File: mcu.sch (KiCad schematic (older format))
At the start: 12 parts, among them J501 JTAG, J502 Serial / Bootloader, SW501 EVQQ2, SW502 EVQQ2, U501 STM32F405RGTx, Y501 8MHz

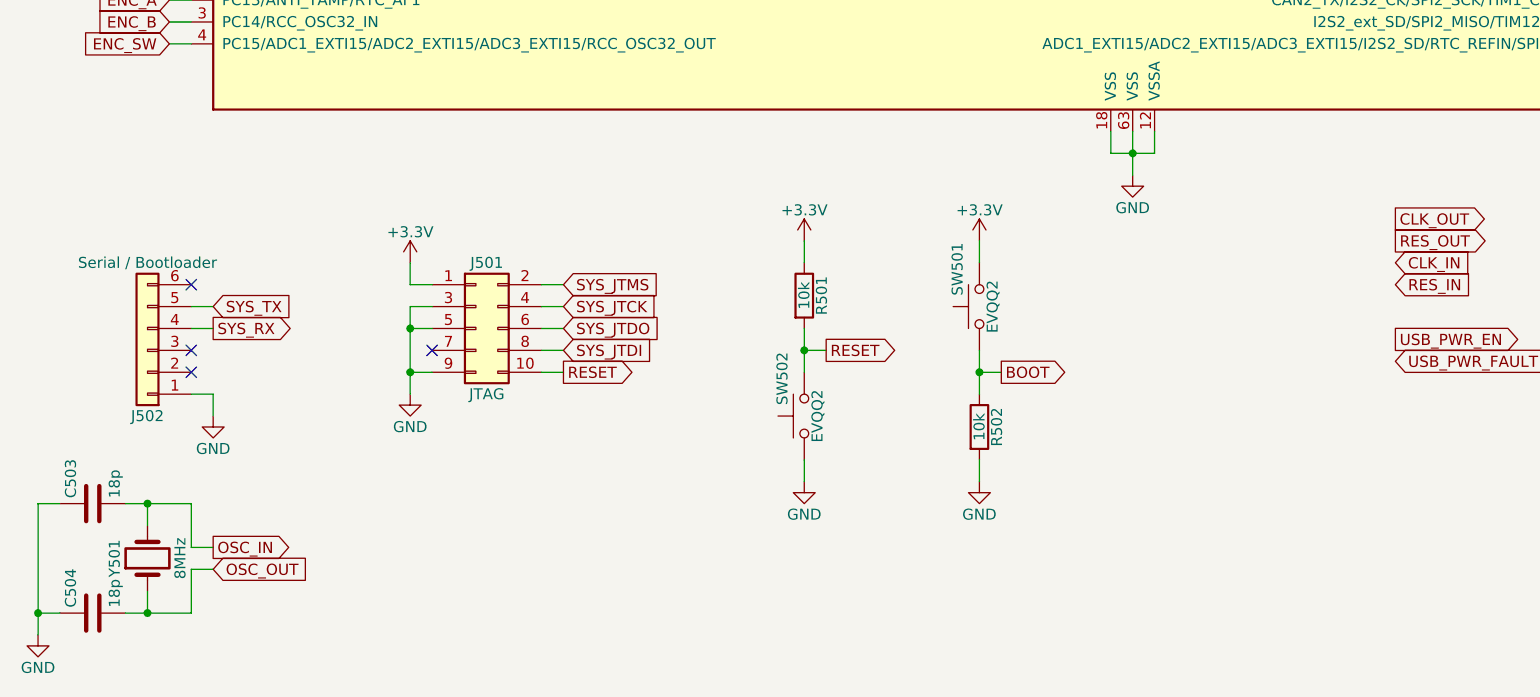
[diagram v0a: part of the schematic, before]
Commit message: work in progress
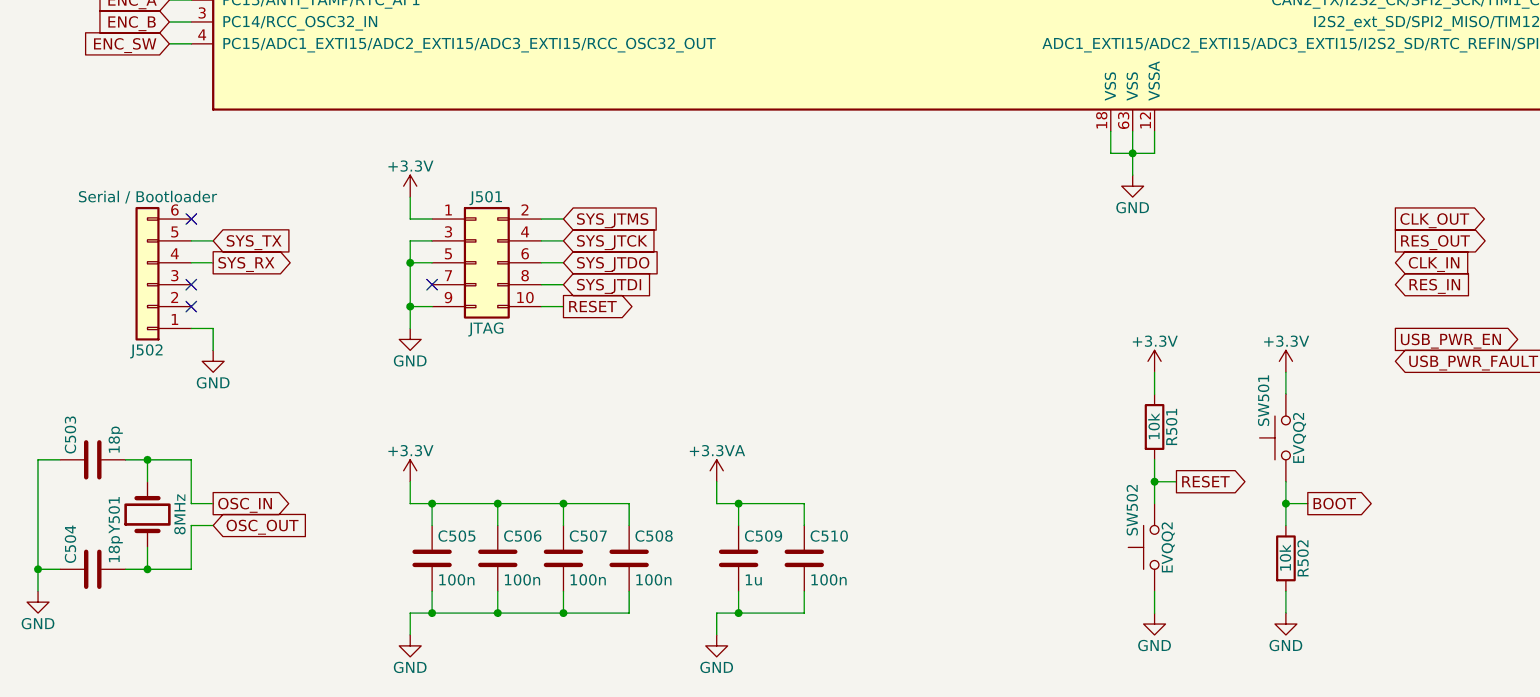
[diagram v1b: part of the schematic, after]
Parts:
- added C505, C506, C507, C508, C510: 100n, Capacitors_SMD:C_0603, symbol C
- added C509: 1u, Capacitors_SMD:C_0603, symbol C
- C501, C502: MFN (none) -> TDK; MFP (none) -> C2012X5R1A225K085AA
- C503, C504: MFN (none) -> Murata; MFP (none) -> GRM1885C1H180JA01J
- R501, R502: MFN (none) -> Panasonic; MFP (none) -> ERJ-3EKF1002V
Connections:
- net +3.3VA: now also C509.1, C510.1
- net +3V3: now also C505.1, C506.1, C507.1, C508.1
- net GND: now also C505.2, C506.2, C507.2, C508.2, C509.2, C510.2
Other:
- moved on the sheet: C503, C504, J501, J502, R501, R502, SW501, SW502, Y501

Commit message: more work
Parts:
- C505, C506, C507, C508, C510: MFN (none) -> Murata; MFP (none) -> GRM188R71E104JA01J
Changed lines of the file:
@@
+	1    0    0    -1
+$EndComp
+$Comp
+L C C505
+U 1 1 59E34530
+P 2600 7150
+F 0 "C505" H 2625 7250 50  0000 L CNN
+F 1 "100n" H 2625 7050 50  0000 L CNN
+F 2 "Capacitors_SMD:C_0603" H 2638 7000 50  0001 C CNN
+F 3 "http://datasheet.octopart.com/GRM188R71E104JA01J-Murata-datasheet-66077098.pdf" H 2600 7150 50  0001 C CNN
+F 4 "Murata" H 2625 7350 50  0001 C CNN "MFN"
+F 5 "GRM188R71E104JA01J" H 2625 7350 50  0001 C CNN "MFP"
+	1    2600 7150
+	1    0    0    -1
+$EndComp
+$Comp
+L C C506
+U 1 1 59E345BC
+P 2900 7150
+F 0 "C506" H 2925 7250 50  0000 L CNN
+F 1 "100n" H 2925 7050 50  0000 L CNN
+F 2 "Capacitors_SMD:C_0603" H 2938 7000 50  0001 C CNN
+F 3 "http://datasheet.octopart.com/GRM188R71E104JA01J-Murata-datasheet-66077098.pdf" H 2900 7150 50  0001 C CNN
+F 4 "Murata" H 2925 7350 50  0001 C CNN "MFN"
+F 5 "GRM188R71E104JA01J" H 2925 7350 50  0001 C CNN "MFP"
+	1    2900 7150
+	1    0    0    -1
+$EndComp
+$Comp
+L C C507
+U 1 1 59E34607
+P 3200 7150
+F 0 "C507" H 3225 7250 50  0000 L CNN
+F 1 "100n" H 3225 7050 50  0000 L CNN
+F 2 "Capacitors_SMD:C_0603" H 3238 7000 50  0001 C CNN
+F 3 "http://datasheet.octopart.com/GRM188R71E104JA01J-Murata-datasheet-66077098.pdf" H 3200 7150 50  0001 C CNN
+F 4 "Murata" H 3225 7350 50  0001 C CNN "MFN"
+F 5 "GRM188R71E104JA01J" H 3225 7350 50  0001 C CNN "MFP"
+	1    3200 7150
+	1    0    0    -1
+$EndComp
+$Comp
+L C C508
+U 1 1 59E34648
+P 3500 7150
+F 0 "C508" H 3525 7250 50  0000 L CNN
+F 1 "100n" H 3525 7050 50  0000 L CNN
+F 2 "Capacitors_SMD:C_0603" H 3538 7000 50  0001 C CNN
+F 3 "http://datasheet.octopart.com/GRM188R71E104JA01J-Murata-datasheet-66077098.pdf" H 3500 7150 50  0001 C CNN
+F 4 "Murata" H 3525 7350 50  0001 C CNN "MFN"
+F 5 "GRM188R71E104JA01J" H 3525 7350 50  0001 C CNN "MFP"
+	1    3500 7150
+	1    0    0    -1
+$EndComp
+$Comp
+L +3.3V #PWR061
+U 1 1 59E34B90
+P 2500 6800
+F 0 "#PWR061" H 2500 6650 50  0001 C CNN
+F 1 "+3.3V" H 2500 6940 50  0000 C CNN
+F 2 "" H 2500 6800 50  0001 C CNN
+F 3 "" H 2500 6800 50  0001 C CNN
+	1    2500 6800
+	1    0    0    -1
+$EndComp
+$Comp
+L GND #PWR062
+U 1 1 59E34BD4
+P 2500 7500
+F 0 "#PWR062" H 2500 7250 50  0001 C CNN
+F 1 "GND" H 2500 7350 50  0000 C CNN
+F 2 "" H 2500 7500 50  0001 C CNN
+F 3 "" H 2500 7500 50  0001 C CNN
+	1    2500 7500
+	1    0    0    -1
+$EndComp
+$Comp
+L +3.3VA #PWR063
+U 1 1 59E35078
+P 3900 6800
+F 0 "#PWR063" H 3900 6650 50  0001 C CNN
+F 1 "+3.3VA" H 3900 6940 50  0000 C CNN
+F 2 "" H 3900 6800 50  0001 C CNN
+F 3 "" H 3900 6800 50  0001 C CNN
+	1    3900 6800
+	1    0    0    -1
+$EndComp
+$Comp
+L GND #PWR064
+U 1 1 59E350BC
+P 3900 7500
+F 0 "#PWR064" H 3900 7250 50  0001 C CNN
+F 1 "GND" H 3900 7350 50  0000 C CNN
+F 2 "" H 3900 7500 50  0001 C CNN
+F 3 "" H 3900 7500 50  0001 C CNN
+	1    3900 7500
+	1    0    0    -1
+$EndComp
+$Comp
+L C C509
+U 1 1 59E35219
+P 4000 7150
+F 0 "C509" H 4025 7250 50  0000 L CNN
+F 1 "1u" H 4025 7050 50  0000 L CNN
+F 2 "Capacitors_SMD:C_0603" H 4038 7000 50  0001 C CNN
+F 3 "" H 4000 7150 50  0001 C CNN
+	1    4000 7150
+	1    0    0    -1
+$EndComp
+$Comp
+L C C510
+U 1 1 59E3526B
+P 4300 7150
+F 0 "C510" H 4325 7250 50  0000 L CNN
+F 1 "100n" H 4325 7050 50  0000 L CNN
+F 2 "Capacitors_SMD:C_0603" H 4338 7000 50  0001 C CNN
+F 3 "http://datasheet.octopart.com/GRM188R71E104JA01J-Murata-datasheet-66077098.pdf" H 4300 7150 50  0001 C CNN
+F 4 "Murata" H 4325 7350 50  0001 C CNN "MFN"
+F 5 "GRM188R71E104JA01J" H 4325 7350 50  0001 C CNN "MFP"
+	1    4300 7150
 	1    0    0    -1
 $EndComp
@@
 Wire Wire Line
 	10100 2800 10200 2800
+Wire Wire Line
+	2500 6900 3500 6900
+Wire Wire Line
+	2600 6900 2600 7000
+Wire Wire Line
+	2900 6900 2900 7000
+Wire Wire Line
+	3200 6900 3200 7000
+Wire Wire Line
+	3500 6900 3500 7000
+Wire Wire Line
+	2500 6900 2500 6800
+Wire Wire Line
+	2500 7400 3500 7400
+Wire Wire Line
+	2600 7400 2600 7300
+Wire Wire Line
+	2900 7400 2900 7300
+Wire Wire Line
+	3500 7400 3500 7300
+Wire Wire Line
+	3200 7300 3200 7400
+Wire Wire Line
+	2500 7400 2500 7500
+Wire Wire Line
+	3900 7500 3900 7400
+Wire Wire Line
+	3900 7400 4300 7400
+Wire Wire Line
+	4000 7400 4000 7300
+Wire Wire Line
+	3900 6800 3900 6900
+Wire Wire Line
+	3900 6900 4300 6900
+Wire Wire Line
+	4000 6900 4000 7000
+Wire Wire Line
+	4300 6900 4300 7000
+Wire Wire Line
+	4300 7400 4300 7300
 Connection ~ 2500 6000
 Connection ~ 2500 5800
@@
 Connection ~ 5900 6800
 Connection ~ 6500 6900
+Connection ~ 2600 6900
+Connection ~ 2900 6900
+Connection ~ 3200 6900
+Connection ~ 2600 7400
+Connection ~ 2900 7400
+Connection ~ 3200 7400
+Connection ~ 4000 6900
+Connection ~ 4000 7400
 NoConn ~ 1500 5600
 NoConn ~ 1500 5900
@@
 NoConn ~ 2600 5900
 NoConn ~ 1500 2000
-$Comp
-L C C505
-U 1 1 59E34530
-P 2600 7150
-F 0 "C505" H 2625 7250 50  0000 L CNN
-F 1 "100n" H 2625 7050 50  0000 L CNN
-F 2 "Capacitors_SMD:C_0603" H 2638 7000 50  0001 C CNN
-F 3 "" H 2600 7150 50  0001 C CNN
-	1    2600 7150
-	1    0    0    -1
-$EndComp
-$Comp
-L C C506
-U 1 1 59E345BC
-P 2900 7150
-F 0 "C506" H 2925 7250 50  0000 L CNN
-F 1 "100n" H 2925 7050 50  0000 L CNN
-F 2 "Capacitors_SMD:C_0603" H 2938 7000 50  0001 C CNN
-F 3 "" H 2900 7150 50  0001 C CNN
-	1    2900 7150
-	1    0    0    -1
-$EndComp
-$Comp
-L C C507
-U 1 1 59E34607
-P 3200 7150
-F 0 "C507" H 3225 7250 50  0000 L CNN
-F 1 "100n" H 3225 7050 50  0000 L CNN
-F 2 "Capacitors_SMD:C_0603" H 3238 7000 50  0001 C CNN
-F 3 "" H 3200 7150 50  0001 C CNN
-	1    3200 7150
-	1    0    0    -1
-$EndComp
-$Comp
-L C C508
-U 1 1 59E34648
-P 3500 7150
-F 0 "C508" H 3525 7250 50  0000 L CNN
-F 1 "100n" H 3525 7050 50  0000 L CNN
-F 2 "Capacitors_SMD:C_0603" H 3538 7000 50  0001 C CNN
-F 3 "" H 3500 7150 50  0001 C CNN
-	1    3500 7150
-	1    0    0    -1
-$EndComp
-Wire Wire Line
-	2500 6900 3500 6900
-Wire Wire Line
-	2600 6900 2600 7000
-Wire Wire Line
-	2900 6900 2900 7000
-Connection ~ 2600 6900
-Wire Wire Line
-	3200 6900 3200 7000
-Connection ~ 2900 6900
-Wire Wire Line
-	3500 6900 3500 7000
-Connection ~ 3200 6900
-Wire Wire Line
-	2500 6900 2500 6800
-Wire Wire Line
-	2500 7400 3500 7400
-Wire Wire Line
-	2600 7400 2600 7300
-Wire Wire Line
-	2900 7400 2900 7300
-Connection ~ 2600 7400
-Wire Wire Line
-	3500 7400 3500 7300
-Connection ~ 2900 7400
-Wire Wire Line
-	3200 7300 3200 7400
-Connection ~ 3200 7400
-Wire Wire Line
-	2500 7400 2500 7500
-$Comp
-L +3.3V #PWR061
-U 1 1 59E34B90
-P 2500 6800
-F 0 "#PWR061" H 2500 6650 50  0001 C CNN
-F 1 "+3.3V" H 2500 6940 50  0000 C CNN
-F 2 "" H 2500 6800 50  0001 C CNN
-F 3 "" H 2500 6800 50  0001 C CNN
-	1    2500 6800
-	1    0    0    -1
-$EndComp
-$Comp
-L GND #PWR062
-U 1 1 59E34BD4
-P 2500 7500
-F 0 "#PWR062" H 2500 7250 50  0001 C CNN
-F 1 "GND" H 2500 7350 50  0000 C CNN
-F 2 "" H 2500 7500 50  0001 C CNN
-F 3 "" H 2500 7500 50  0001 C CNN
-	1    2500 7500
-	1    0    0    -1
-$EndComp
-$Comp
-L +3.3VA #PWR063
-U 1 1 59E35078
-P 3900 6800
-F 0 "#PWR063" H 3900 6650 50  0001 C CNN
-F 1 "+3.3VA" H 3900 6940 50  0000 C CNN
-F 2 "" H 3900 6800 50  0001 C CNN
-F 3 "" H 3900 6800 50  0001 C CNN
-	1    3900 6800
-	1    0    0    -1
-$EndComp
-$Comp
-L GND #PWR064
-U 1 1 59E350BC
-P 3900 7500
-F 0 "#PWR064" H 3900 7250 50  0001 C CNN
-F 1 "GND" H 3900 7350 50  0000 C CNN
-F 2 "" H 3900 7500 50  0001 C CNN
-F 3 "" H 3900 7500 50  0001 C CNN
-	1    3900 7500
-	1    0    0    -1
-$EndComp
-Wire Wire Line
-	3900 7500 3900 7400
-Wire Wire Line
-	3900 7400 4300 7400
-Wire Wire Line
-	4000 7400 4000 7300
-Wire Wire Line
-	3900 6800 3900 6900
-Wire Wire Line
-	3900 6900 4300 6900
-Wire Wire Line
-	4000 6900 4000 7000
-$Comp
-L C C509
-U 1 1 59E35219
-P 4000 7150
-F 0 "C509" H 4025 7250 50  0000 L CNN
-F 1 "1u" H 4025 7050 50  0000 L CNN
-F 2 "Capacitors_SMD:C_0603" H 4038 7000 50  0001 C CNN
-F 3 "" H 4000 7150 50  0001 C CNN
-	1    4000 7150
-	1    0    0    -1
-$EndComp
-$Comp
-L C C510
-U 1 1 59E3526B
-P 4300 7150
-F 0 "C510" H 4325 7250 50  0000 L CNN
-F 1 "100n" H 4325 7050 50  0000 L CNN
-F 2 "Capacitors_SMD:C_0603" H 4338 7000 50  0001 C CNN
-F 3 "" H 4300 7150 50  0001 C CNN
-	1    4300 7150
-	1    0    0    -1
-$EndComp
-Wire Wire Line
-	4300 6900 4300 7000
-Connection ~ 4000 6900
-Wire Wire Line
-	4300 7400 4300 7300
-Connection ~ 4000 7400
 $EndSCHEMATC
